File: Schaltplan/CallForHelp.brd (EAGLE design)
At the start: 109.6 x 86 mm, 20 parts

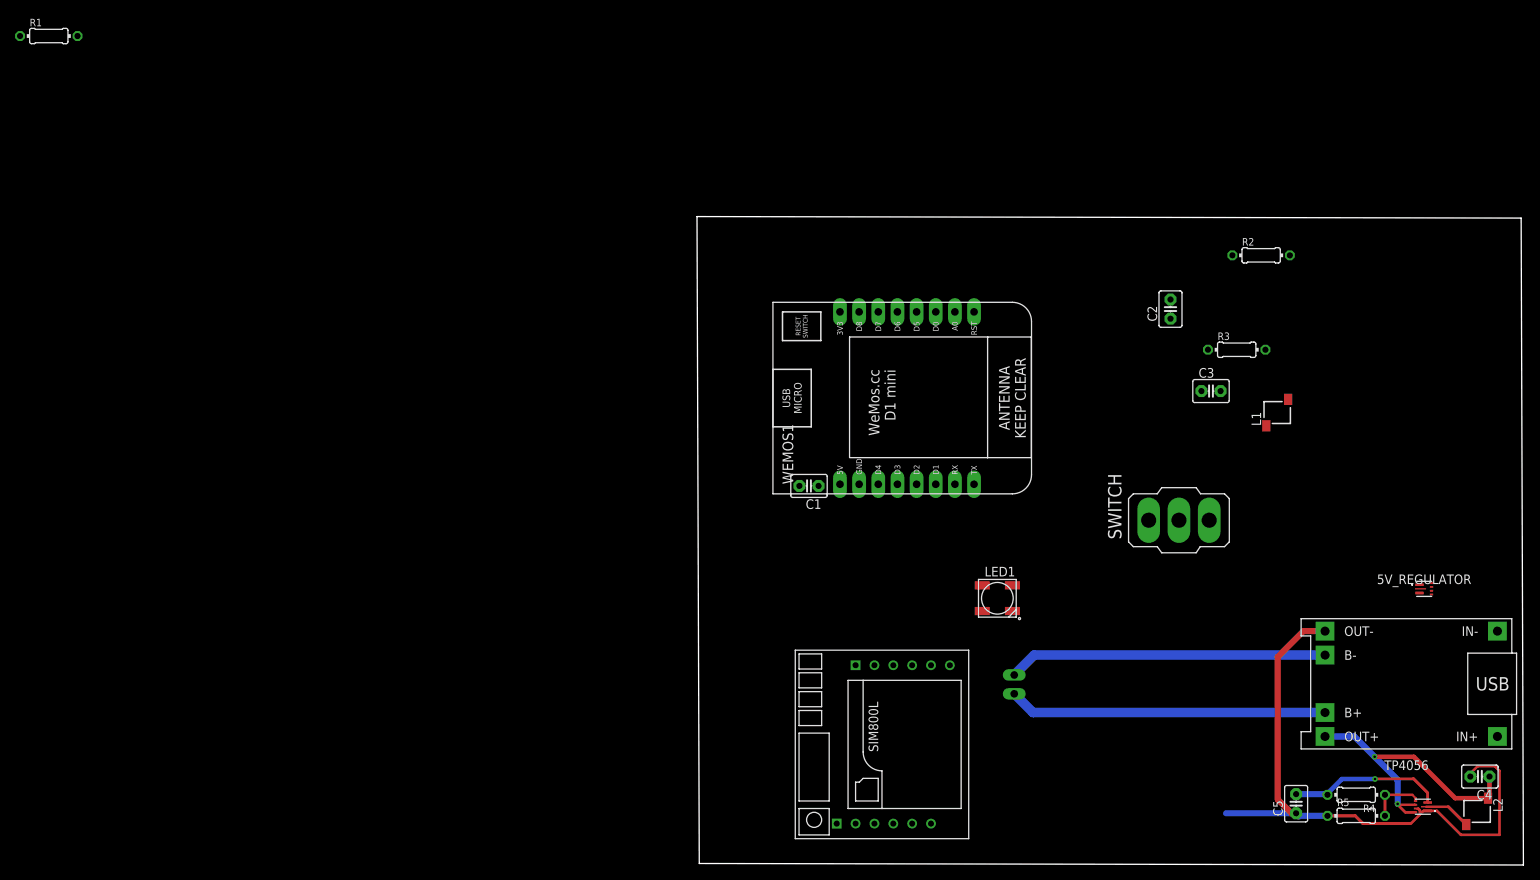
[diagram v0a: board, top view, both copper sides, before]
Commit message: Board finished
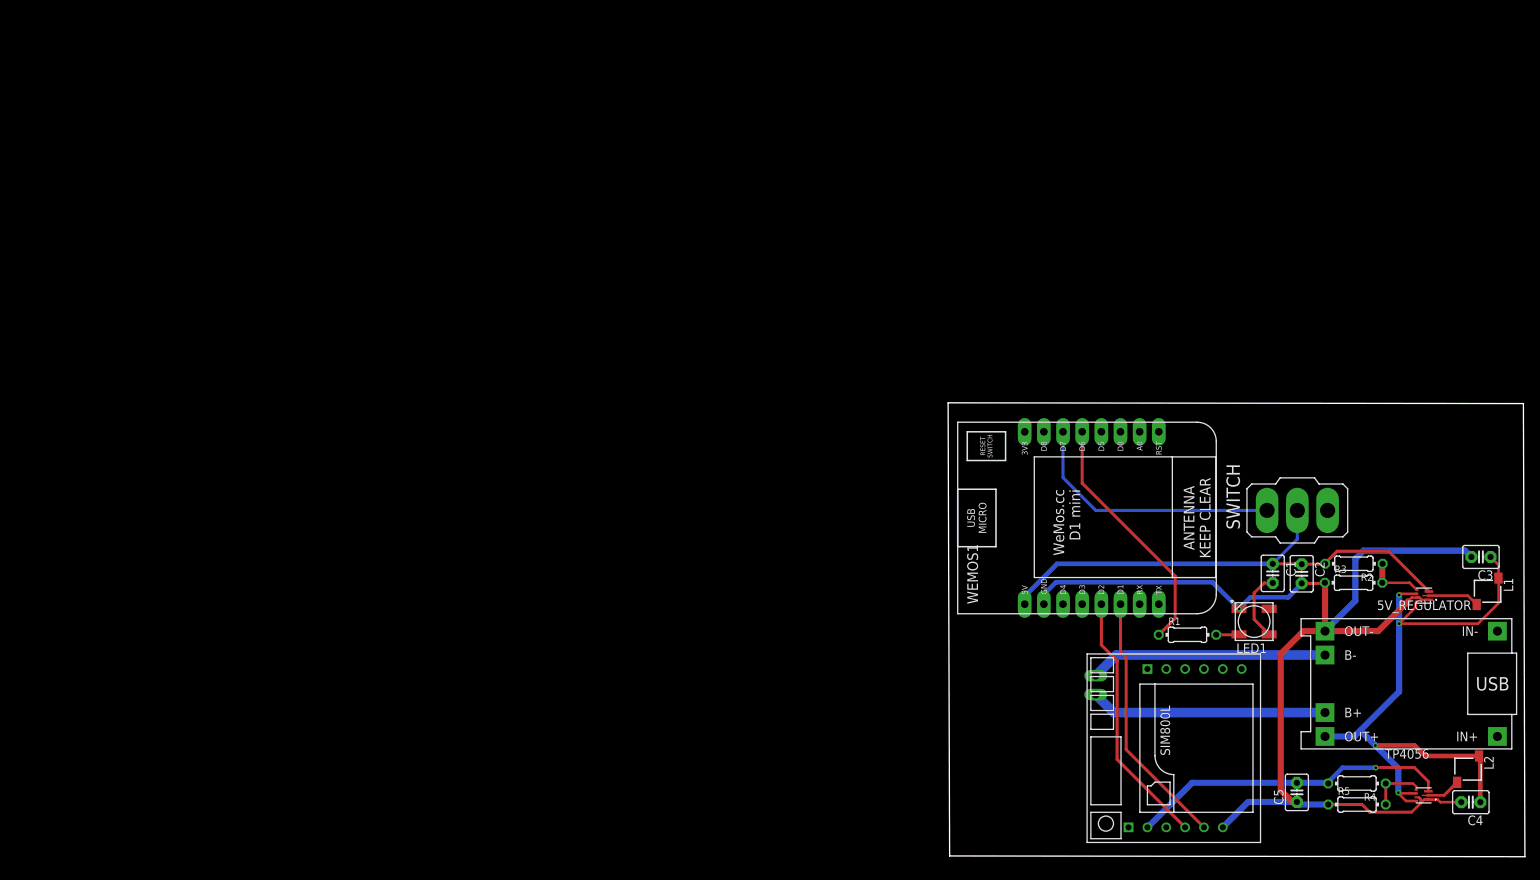
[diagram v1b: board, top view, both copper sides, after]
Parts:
- C5: value 10uF -> 33uF
- R2: value 100kΩ -> 732kΩ
- R3, R5: value 732kΩ -> 100kΩ
- R4: value 100kΩ -> 604kΩ
- moved R1 170.6 mm to (22.7, 20.9)
- moved C1 62.6 mm to (34.0, 29.1), turned to 270 degrees
- moved R2 42.7 mm to (44.8, 30.4), turned to 180 degrees
- moved C3 42.0 mm to (61.6, 31.2), turned to 180 degrees
- moved C2 39.2 mm to (37.9, 29.0), turned to 270 degrees
- moved SIM800L 38.7 mm to (20.9, 5.89)
- moved L1 36.6 mm to (62.5, 26.7), turned to 180 degrees
- moved R3 34.6 mm to (44.8, 27.8)
- moved LED1 34.2 mm to (31.6, 22.7), turned to 180 degrees
- moved WEMOS1 29.2 mm to (11.3, 37.7)
- moved SWITCH 15.8 mm to (37.3, 37.4)
- moved BATTERIE 10.8 mm to (16.8, 14.2)
- moved L2 5.73 mm to (59.9, 3.11)
- moved C4 3.61 mm to (60.3, -1.27)
- moved C5 1.50 mm to (37.2, 0.03)
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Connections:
- removed net N$12: SIM800L.RST, SIM800L.VCC
- net VCC: now also SIM800L.VCC
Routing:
- net GND: track 83.0 -> 155.1 mm, vias 0 -> 1
- net +5V: track 0.00 -> 67.9 mm
- net V+: track 40.8 -> 89.0 mm, vias 2 -> 4
- net N$8: track 0.00 -> 34.9 mm
- net N$6: track 0.00 -> 34.2 mm
- net N$7: track 0.00 -> 34.2 mm
- net LED_PIN: track 0.00 -> 32.9 mm
- net VCC: track 20.5 -> 42.8 mm
- net BATTERY_VCC: track 42.2 -> 31.4 mm
- net BATTERY_GND: track 42.3 -> 31.5 mm
- net N$11: track 0.00 -> 9.34 mm
- net N$2: track 0.00 -> 7.85 mm
- net N$10: track 0.00 -> 6.97 mm
- net N$3: track 0.00 -> 3.05 mm
- net N$9: track 6.25 -> 4.68 mm
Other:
- board size 109.6 x 86 mm -> 76.5 x 60.2 mm
